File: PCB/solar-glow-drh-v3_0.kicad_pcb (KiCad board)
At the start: 2 copper layers, 50.8 x 88.9 mm, 54 parts, among them J1 UPDI hdr, Q1 BCP5316MTWG, SW2 LED master, U1 AVR64DD28 (VQFN28), U2 ALD910025SALI, U3 LIS2DH12, U4 TLV431BCDBZR, U5 NT3H2211, U6 TPS22918

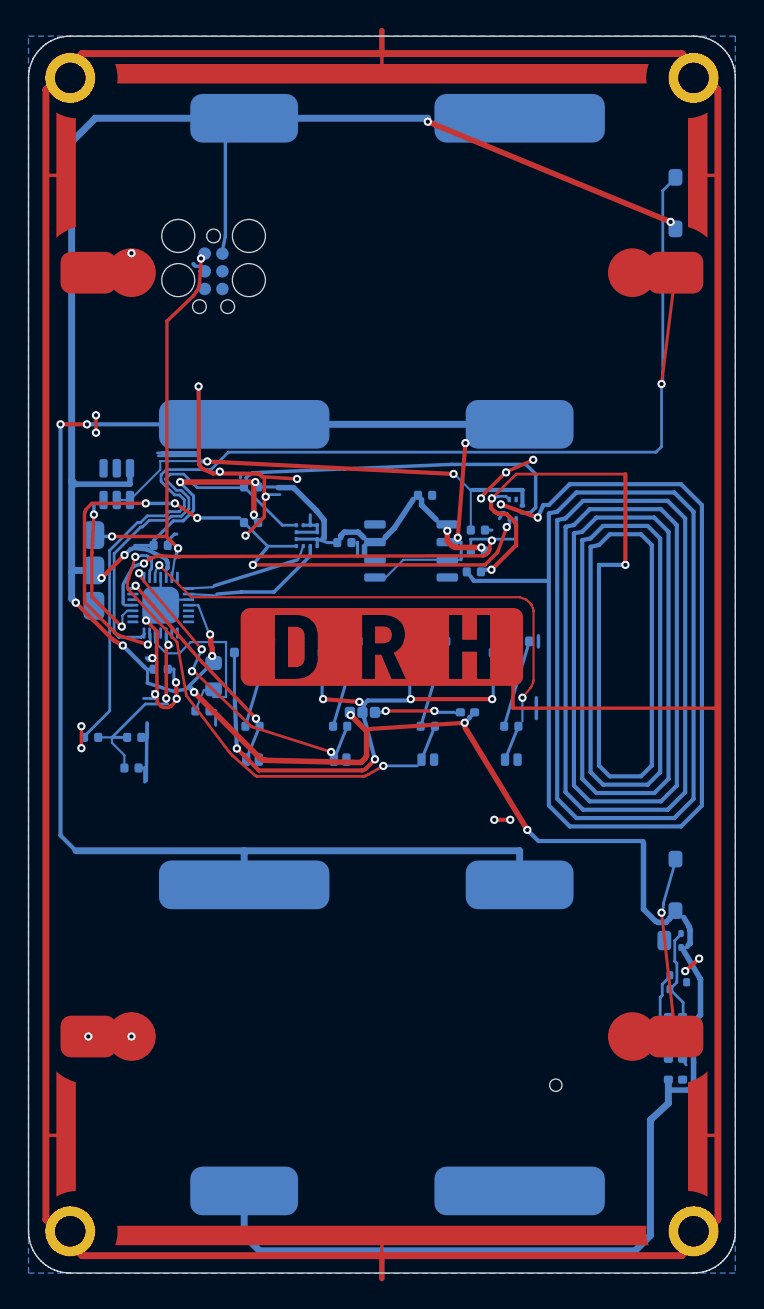
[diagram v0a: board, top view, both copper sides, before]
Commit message: Add files via upload
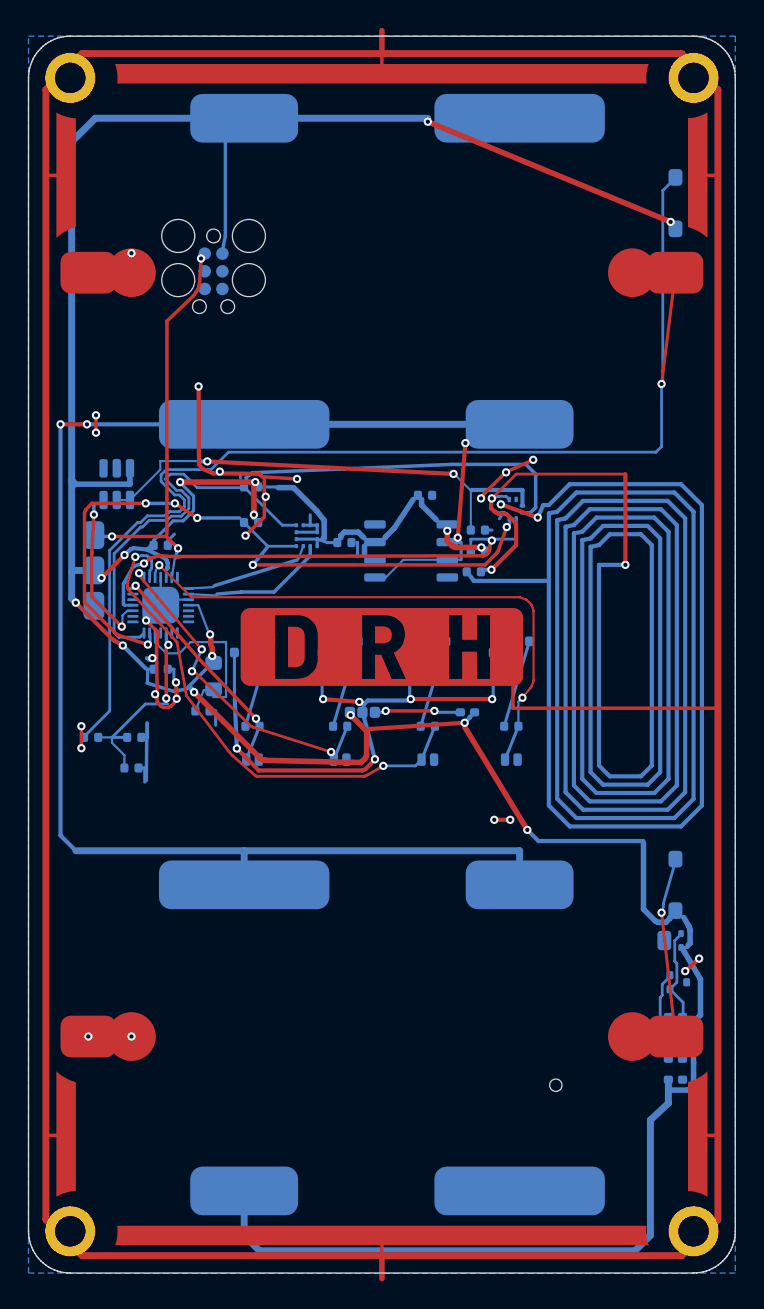
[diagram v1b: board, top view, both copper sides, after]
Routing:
- net GND: track 89.2 -> 64.8 mm
- net VS: track 267.9 -> 267.2 mm
- net VSENSE: track 15.5 -> 14.9 mm
